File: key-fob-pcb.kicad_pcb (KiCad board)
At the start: 4 copper layers, 23 parts, among them J1 Programming Header, J2 Programming Jumper, Q1 IRLML6402TRPBF, SW1 START/STOP BTN, SW5 EN, U1 ESP32-S3-MINI-1, U2 TPS61023DRLT, U3 IRLML2502TRPBF

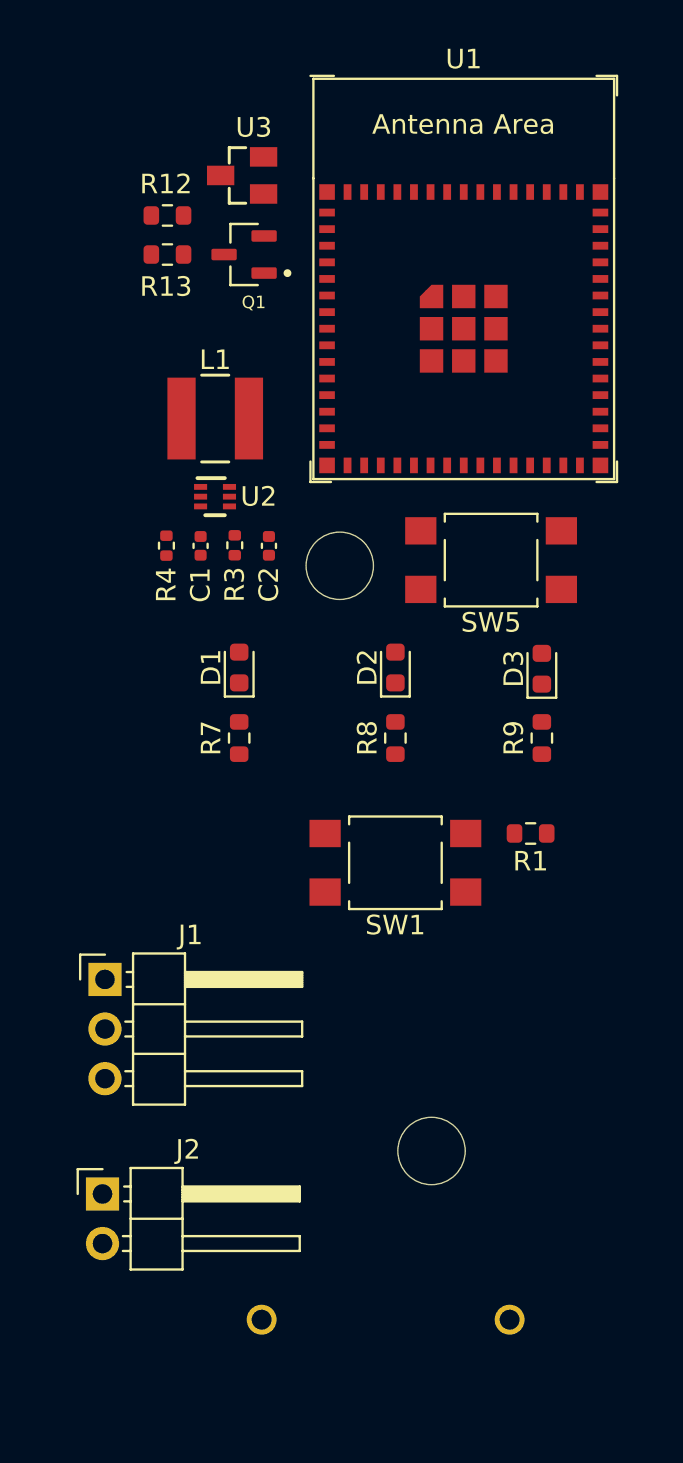
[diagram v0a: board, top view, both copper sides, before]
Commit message: layout complete
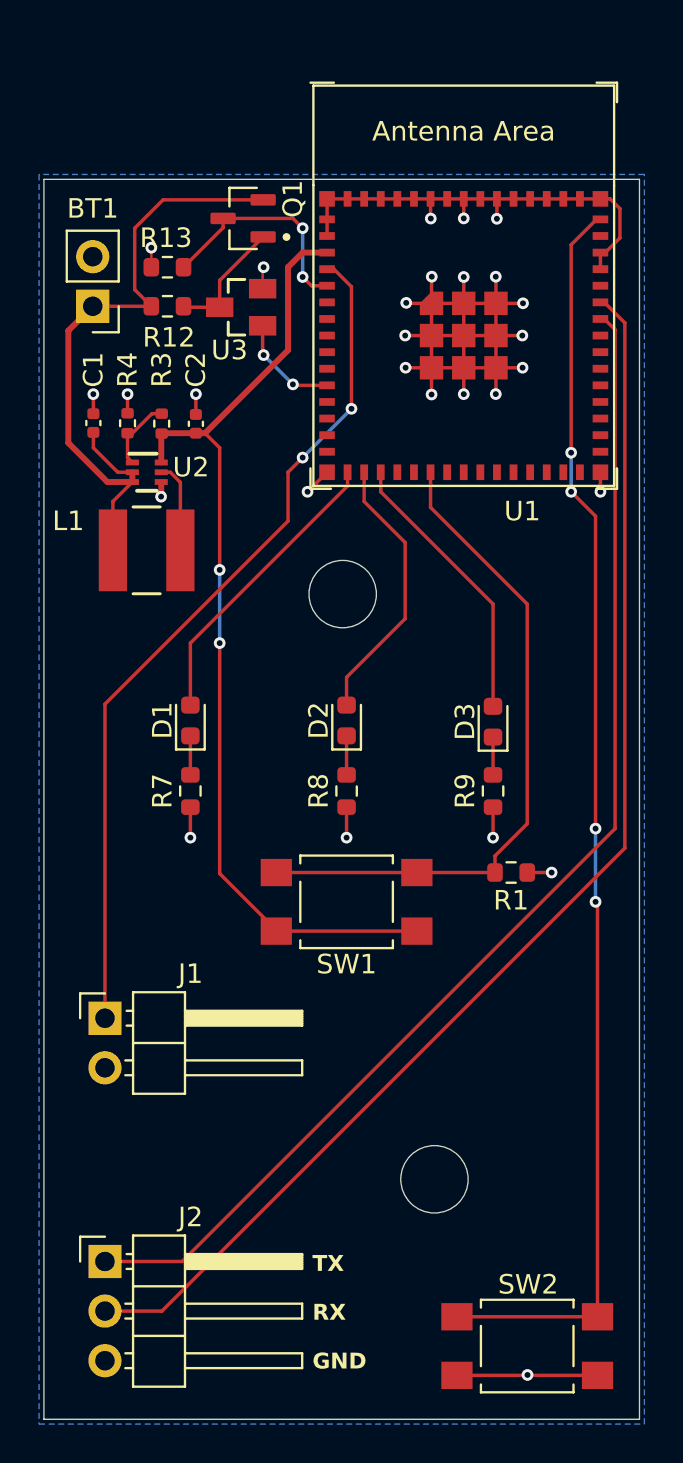
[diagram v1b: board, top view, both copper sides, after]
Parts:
- added Battery Holder: BAT_2468, 2469:BAT_2469, B.Cu at (142.2, 119.0)
- BT1: value 2468 -> AAAx2; footprint 2468:BAT_2468 -> Connector_PinHeader_2.54mm:PinHeader_1x02_P2.54mm_Vertical; moved to F.Cu
- moved SW2 40.3 mm to (149.2, 142.2)
- moved BT1 31.8 mm to (127.0, 89.0), turned to 180 degrees
- moved J2 14.4 mm to (127.6, 137.9)
- moved J1 9.00 mm to (127.6, 125.5)
- moved C1 8.35 mm to (127.0, 95.0), turned to 90 degrees
- moved L1 7.61 mm to (129.8, 101.5), turned to 180 degrees
- moved C2 7.28 mm to (132.3, 95.0), turned to 90 degrees
- moved R3 7.27 mm to (130.5, 95.0), turned to 90 degrees
- moved U3 6.75 mm to (134.6, 89.0)
- moved R4 6.58 mm to (128.8, 95.0), turned to 90 degrees
- moved R12 4.65 mm to (130.8, 89.0), turned to 0 degrees
- moved U2 3.71 mm to (129.8, 97.5)
- moved D1 3.69 mm to (132.0, 110.2)
- moved D2 3.69 mm to (140.0, 110.2)
- moved D3 3.69 mm to (147.5, 110.3)
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- renumbered J2 to J1, J1 to J2, SW5 to SW2
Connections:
- U1 pad 10: /LED2 -> unconnected-(U1-GPIO6/TOUCH6/ADC1_CH5-Pad10)
- U1 pad 11: /LED3 -> /VBAT_ADC_EN
- U1 pad 12: /VBAT_ADC_EN -> unconnected-(U1-GPIO8/TOUCH8/ADC1_CH7/SUBSPICS1-Pad12)
- U1 pad 16: unconnected-(U1-GPIO12/TOUCH12/ADC2_CH1/FSPICLK/FSPIIO6/SUBSPICLK-Pad16) -> /LED1
- U1 pad 17: unconnected-(U1-GPIO13/TOUCH13/ADC2_CH2/FSPIQ/FSPIIO7/SUBSPIQ-Pad17) -> /LED2
- U1 pad 18: unconnected-(U1-GPIO14/TOUCH14/ADC2_CH3/FSPIWP/FSPIDQS/SUBSPIWP-Pad18) -> /LED3
- U1 pad 21: unconnected-(U1-GPIO17/U1TXD/ADC2_CH6-Pad21) -> /START_STOP
- U1 pad 8: /START_STOP -> unconnected-(U1-GPIO4/TOUCH4/ADC1_CH3-Pad8)
- U1 pad 9: /LED1 -> unconnected-(U1-GPIO5/TOUCH5/ADC1_CH4-Pad9)
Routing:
- net /ADC/GND: track 0.00 -> 81.3 mm, vias 0 -> 28
- net /RX: track 0.00 -> 65.0 mm
- net /EN: track 0.00 -> 64.8 mm, vias 0 -> 4
- net /TX: track 0.00 -> 61.8 mm
- net /VCC: track 0.00 -> 50.5 mm, vias 0 -> 2
- net /BOOT: track 0.00 -> 44.3 mm, vias 0 -> 2
- net /ADC/VIN: track 0.00 -> 34.8 mm
- net /START_STOP: track 0.00 -> 34.4 mm
- net /LED1: track 0.00 -> 15.3 mm
- net /LED3: track 0.00 -> 14.4 mm
- net /LED2: track 0.00 -> 14.0 mm
- net /VBAT_ADC: track 0.00 -> 11.6 mm, vias 0 -> 2
- net Net-(Q1-Pad1): track 0.00 -> 7.32 mm
- net /VBAT_ADC_EN: track 0.00 -> 5.46 mm, vias 0 -> 2
- net Net-(U2-SW): track 0.00 -> 4.68 mm
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- added copper zone on B.Cu, net /ADC/GND
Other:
- board outline added: 30.5 x 63.5 mm
- copper layers 4 -> 2
- board text added: "+"
- board text added: "-"
- board text added: "Ben Martens 2023-11"
- board text added: "GND"
- board text added: "RX"
- board text added: "TX"
